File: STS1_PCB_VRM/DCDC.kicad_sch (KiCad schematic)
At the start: 25 parts, among them Q2 BSS123, U6 MP28167GQ

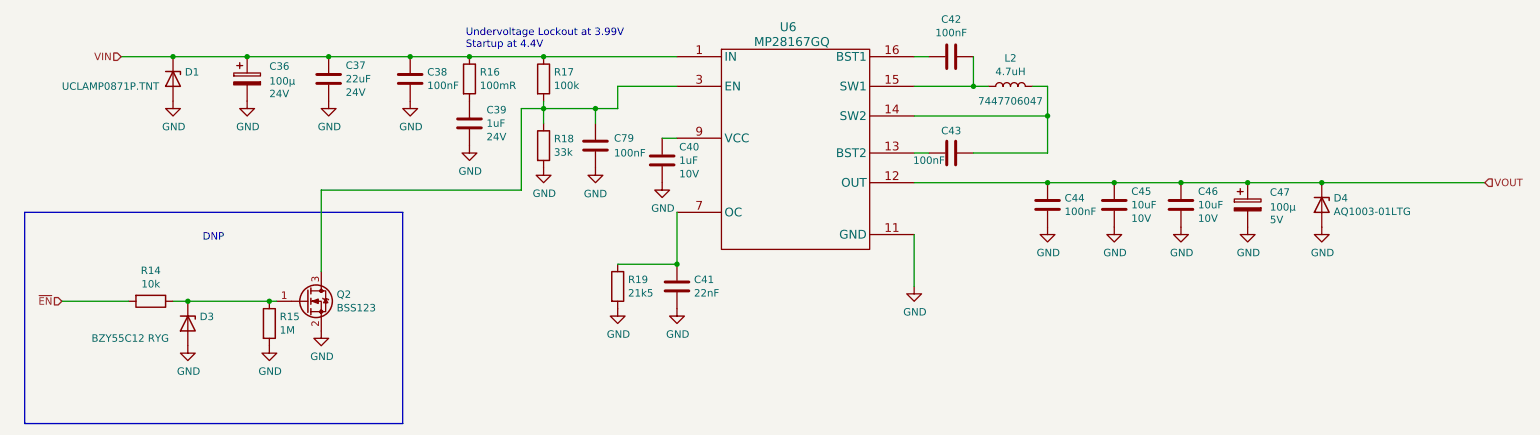
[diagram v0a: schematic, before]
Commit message: feat: more schematic cleanup
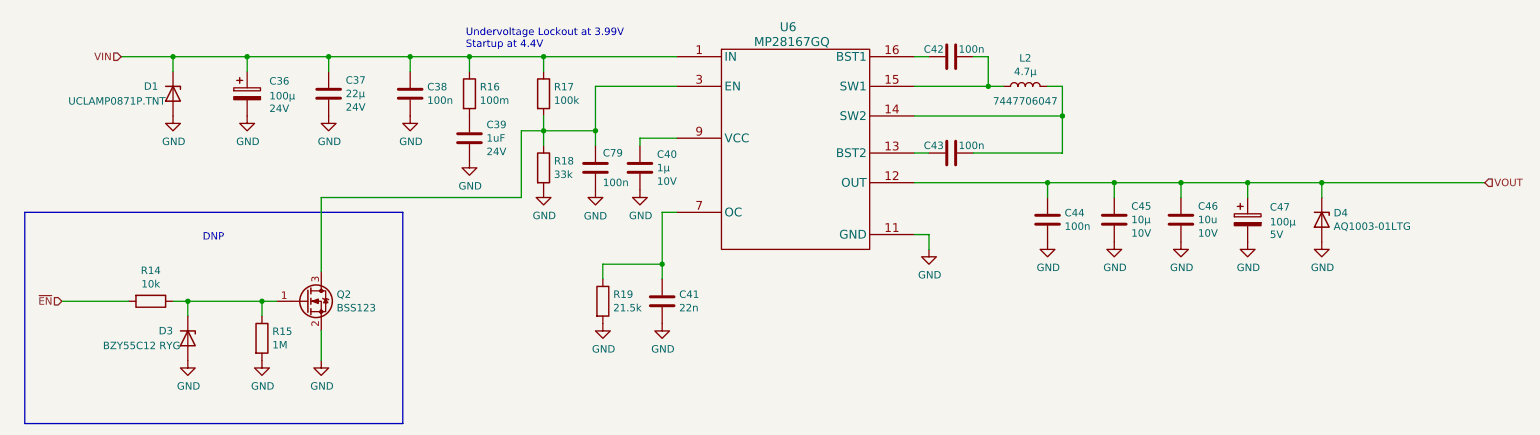
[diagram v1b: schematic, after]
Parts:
- C37: value 22uF -> 22µ
- C38, C42, C43, C44, C79: value 100nF -> 100n
- C40: value 1uF -> 1µ
- C41: value 22nF -> 22n
- C45: value 10uF -> 10µ
- C46: value 10uF -> 10u
- D3, Q2, R14, R15: now left out of the parts list
- L2: value 4.7uH -> 4.7µ
- R16: value 100mR -> 100m
- R19: value 21k5 -> 21.5k
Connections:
- net AGND renamed GND
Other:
- moved on the sheet: C36, C37, C38, C39, C40, C41, C44, C45, C46, C47, C79, D1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

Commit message: feat(RF): better LPF tuning and add part numbers to all inductors
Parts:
- L2: Part 7447706047 -> (none); PartNumber (none) -> 7447706047
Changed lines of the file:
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@@
       (effects (font (size 1.27 1.27)) hide)
     )
-    (property "Part" "7447706047 " (id 4) (at 187.96 68.58 90))
+    (property "PartNumber" "7447706047 " (id 4) (at 187.96 68.58 90))
     (pin "1")
     (pin "2")
